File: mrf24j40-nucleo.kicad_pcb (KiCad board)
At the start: 2 copper layers, 28.6 x 25.4 mm, 2 parts, among them M1 MRF24J40MA_TRANSEIVER_MODULE, P1 CONN_02X08

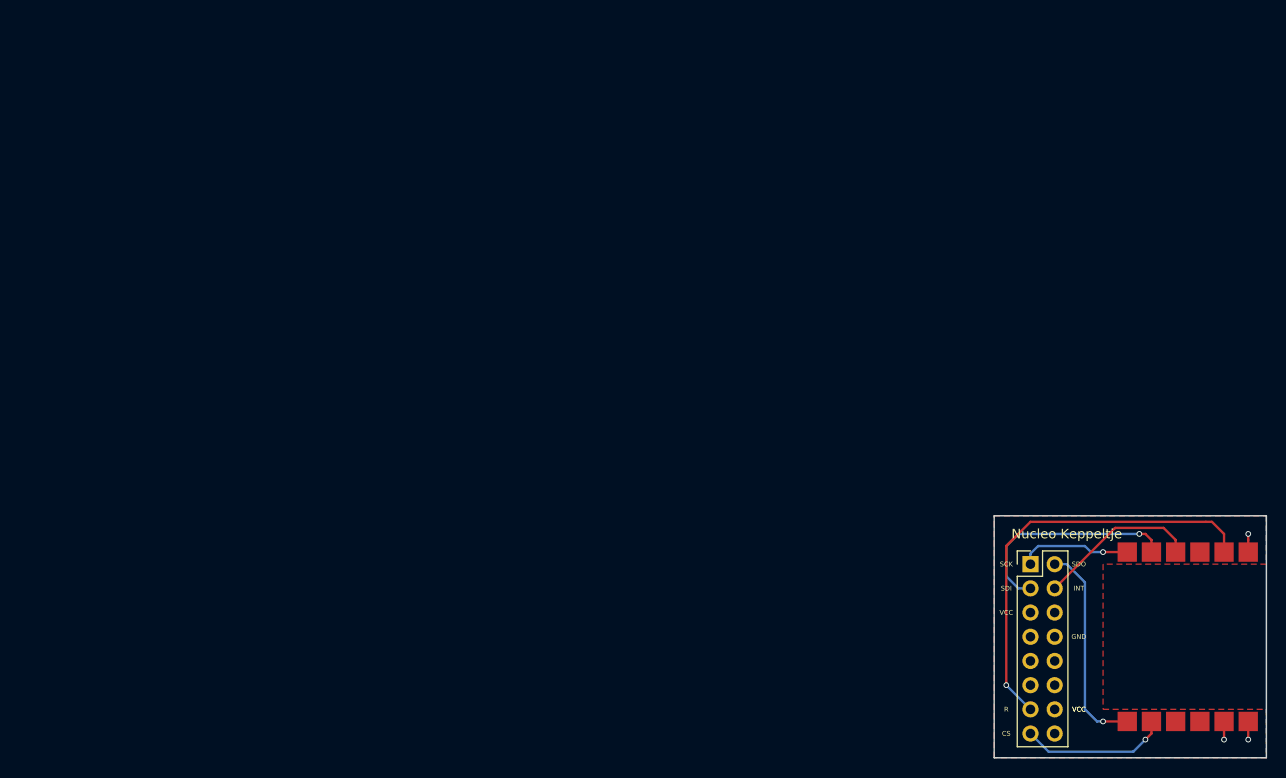
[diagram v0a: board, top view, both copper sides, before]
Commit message: Change sheet size
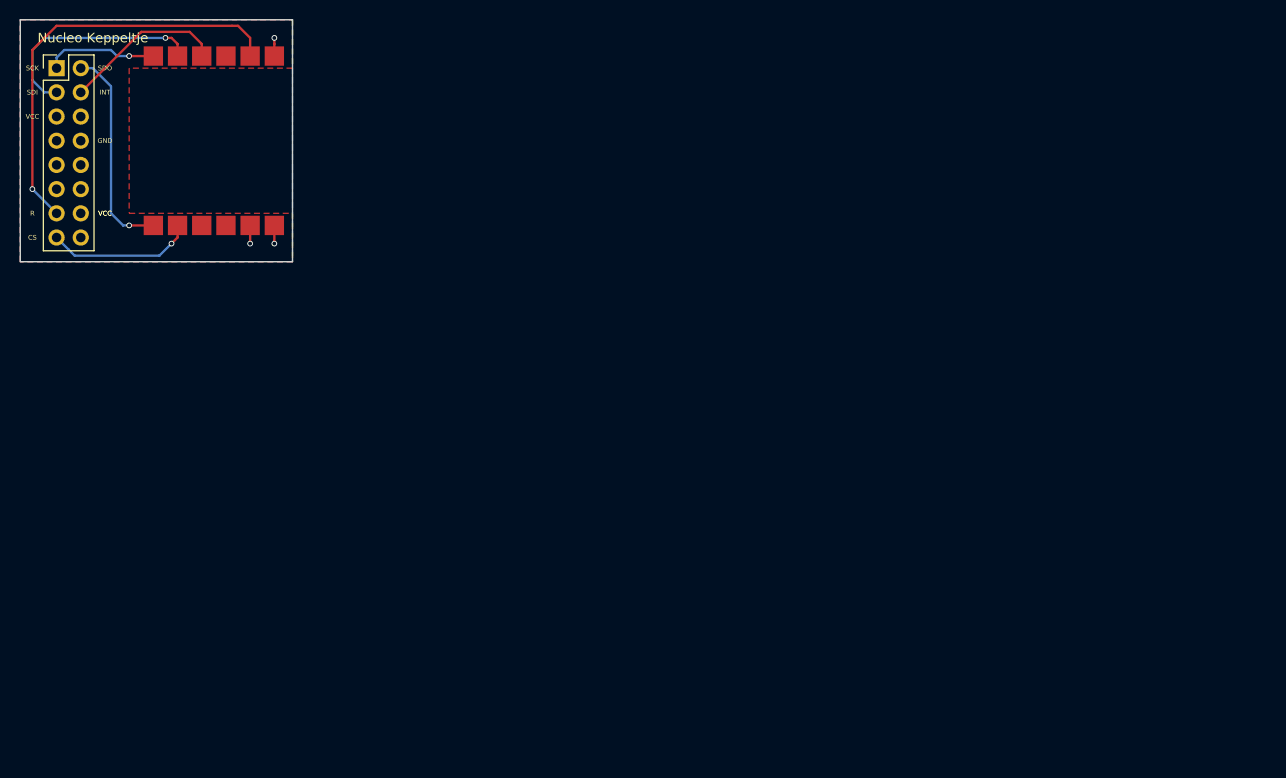
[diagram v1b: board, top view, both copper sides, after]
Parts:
- moved M1 114.7 mm to (95.6, 35.6)
- moved P1 114.7 mm to (87.0, 36.8)
